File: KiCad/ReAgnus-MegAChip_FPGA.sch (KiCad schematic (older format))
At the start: 3 parts, among them J2 Conn_02x05_Odd_Even, U10 AS4C4M16SA, U7 GW1N-UV9LQ144

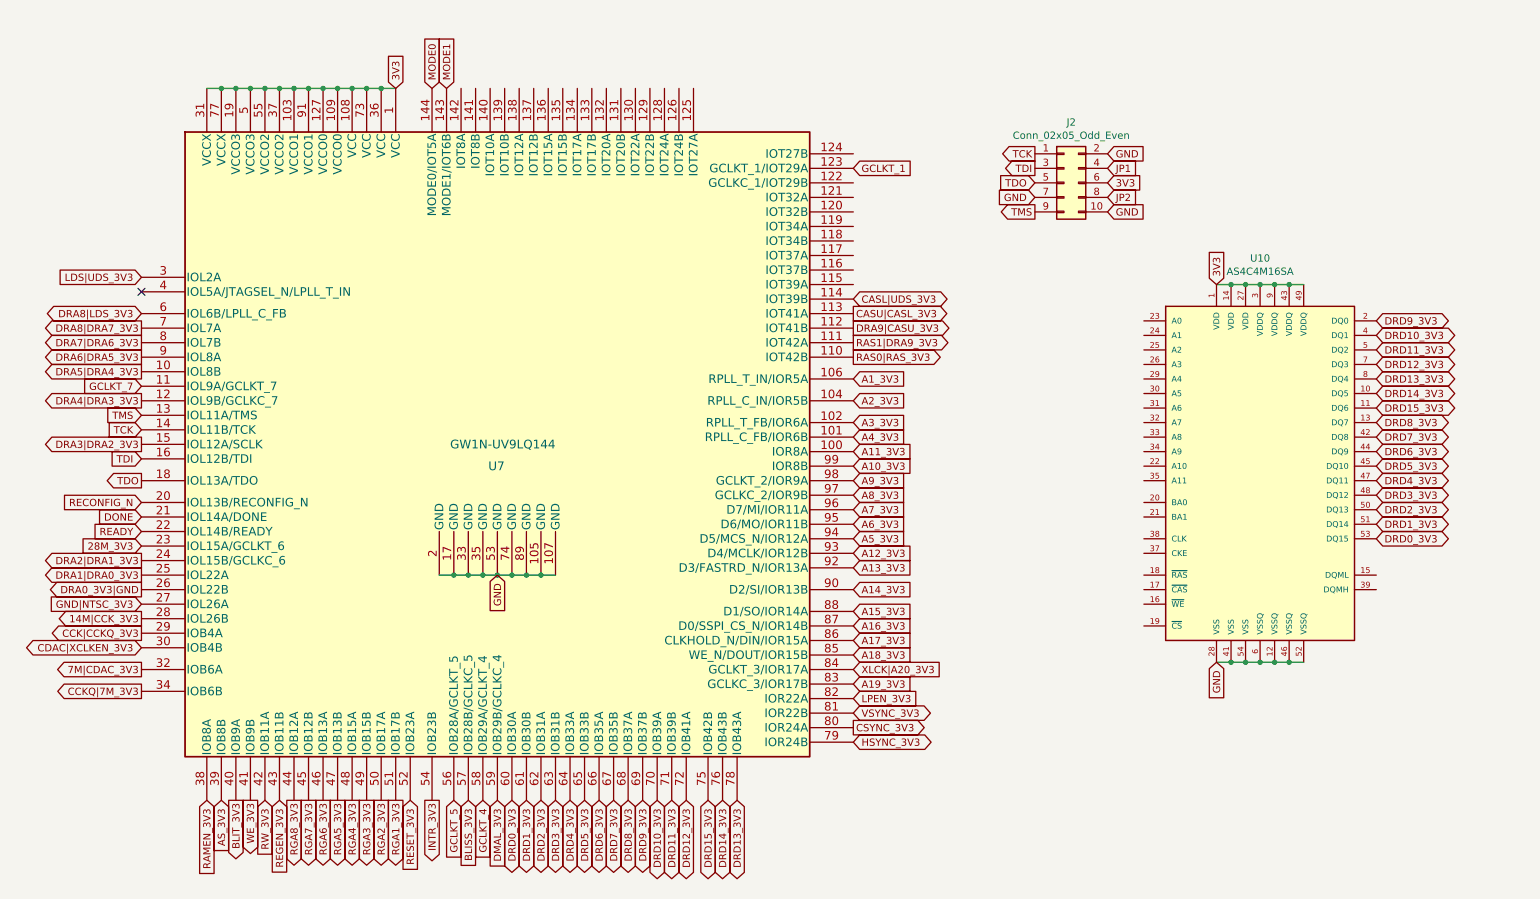
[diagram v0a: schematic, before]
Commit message: more routing and placing components
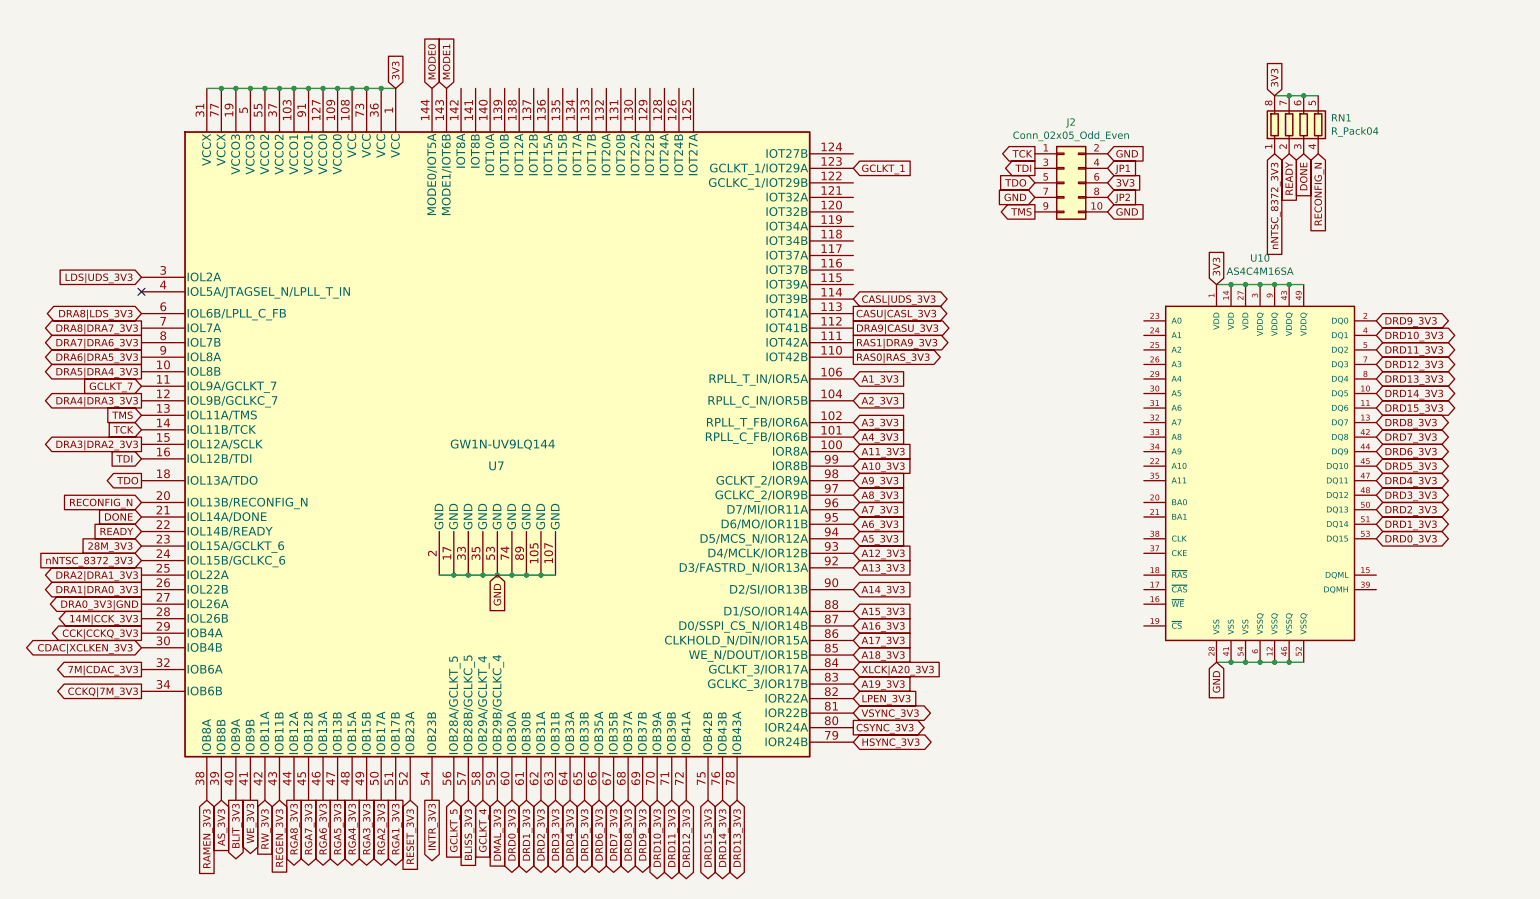
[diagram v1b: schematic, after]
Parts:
- added RN1: R_Pack04, Agnus:RESCAF80P320X160X60-8N, symbol Device:R_Pack04
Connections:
- net GND|NTSC_3V3 is gone; now on net DRA0_3V3|GND: U7.27 (IOL26A)
- net 3V3: now also RN1.5 (R4.2), RN1.6 (R3.2), RN1.7 (R2.2), RN1.8 (R1.2)
- net DONE: now also RN1.3 (R3.1)
- net DRA0_3V3|GND: no longer U7.26 (IOL22B)
- net DRA1|DRA0_3V3: now also U7.26 (IOL22B); no longer U7.25 (IOL22A)
- net DRA2|DRA1_3V3: now also U7.25 (IOL22A); no longer U7.24 (IOL15B/GCLKC_6)
- net READY: now also RN1.2 (R2.1)
- net RECONFIG_N: now also RN1.4 (R4.1)
- new net nNTSC_8372_3V3: RN1.1 (R1.1), U7.24 (IOL15B/GCLKC_6)
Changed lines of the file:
@@
 Text GLabel 5350 5950 3    50   BiDi ~ 0
 DRD15_3V3
-Text GLabel 1450 4600 0    50   Input ~ 0
-GND|NTSC_3V3
 Text GLabel 6350 4950 2    50   Input ~ 0
 A18_3V3
@@
 Text GLabel 1450 3500 0    50   Output ~ 0
 DRA3|DRA2_3V3
-Text GLabel 1450 4300 0    50   Output ~ 0
+Text GLabel 1450 4400 0    50   Output ~ 0
 DRA2|DRA1_3V3
-Text GLabel 1450 4400 0    50   Output ~ 0
+Text GLabel 1450 4500 0    50   Output ~ 0
 DRA1|DRA0_3V3
-Text GLabel 1450 4500 0    50   Output ~ 0
+Text GLabel 1450 4600 0    50   Output ~ 0
 DRA0_3V3|GND
 Text GLabel 2100 5950 3    50   Output ~ 0
@@
 Wire Wire Line
 	9350 5000 9450 5000
+Text GLabel 1450 4300 0    50   Input ~ 0
+nNTSC_8372_3V3
+$Comp
+L Device:R_Pack04 RN1
+U 1 1 6329F720
+P 9450 1300
+F 0 "RN1" H 9638 1346 50  0000 L CNN
+F 1 "R_Pack04" H 9638 1255 50  0000 L CNN
+F 2 "Agnus:RESCAF80P320X160X60-8N" V 9725 1300 50  0001 C CNN
+F 3 "~" H 9450 1300 50  0001 C CNN
+	1    9450 1300
+	1    0    0    -1
+$EndComp
+Text GLabel 9250 1100 1    50   Input ~ 0
+3V3
+Wire Wire Line
+	9250 1100 9350 1100
+Connection ~ 9350 1100
+Wire Wire Line
+	9350 1100 9450 1100
+Connection ~ 9450 1100
+Wire Wire Line
+	9450 1100 9550 1100
+Text GLabel 9550 1500 3    50   Input ~ 0
+RECONFIG_N
+Text GLabel 9450 1500 3    50   Input ~ 0
+DONE
+Text GLabel 9350 1500 3    50   Input ~ 0
+READY
+Text GLabel 9250 1500 3    50   Input ~ 0
+nNTSC_8372_3V3
 $EndSCHEMATC

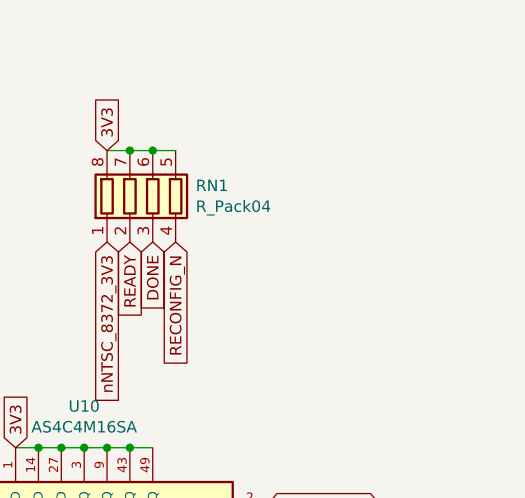
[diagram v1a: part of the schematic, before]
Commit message: more routing and placing components
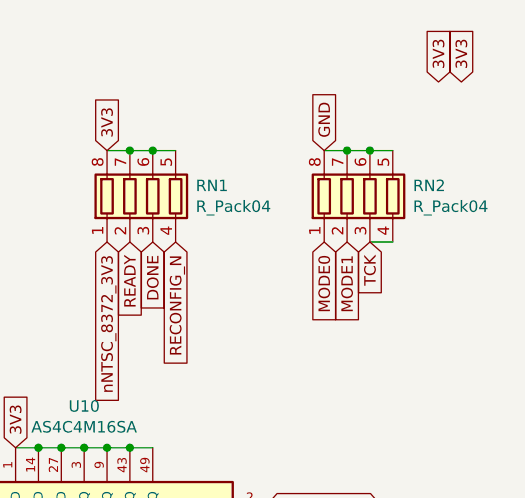
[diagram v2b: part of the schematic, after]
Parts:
- added RN2: R_Pack04, Agnus:RESCAF80P320X160X60-8N, symbol Device:R_Pack04
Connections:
- net GND: now also RN2.5 (R4.2), RN2.6 (R3.2), RN2.7 (R2.2), RN2.8 (R1.2)
- net MODE0: now also RN2.1 (R1.1)
- net MODE1: now also RN2.2 (R2.1)
- net TCK: now also RN2.3 (R3.1), RN2.4 (R4.1)
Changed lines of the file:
@@
 Text GLabel 9250 1500 3    50   Input ~ 0
 nNTSC_8372_3V3
+Text GLabel 10200 1100 1    50   Input ~ 0
+GND
+Text GLabel 10300 1500 3    50   Input ~ 0
+MODE1
+Text GLabel 10200 1500 3    50   Input ~ 0
+MODE0
+Text GLabel 10800 800  1    50   Input ~ 0
+3V3
+$Comp
+L Device:R_Pack04 RN2
+U 1 1 63318369
+P 10400 1300
+F 0 "RN2" H 10588 1346 50  0000 L CNN
+F 1 "R_Pack04" H 10588 1255 50  0000 L CNN
+F 2 "Agnus:RESCAF80P320X160X60-8N" V 10675 1300 50  0001 C CNN
+F 3 "~" H 10400 1300 50  0001 C CNN
+	1    10400 1300
+	1    0    0    -1
+$EndComp
+Text GLabel 10700 800  1    50   Input ~ 0
+3V3
+Wire Wire Line
+	10200 1100 10300 1100
+Connection ~ 10300 1100
+Wire Wire Line
+	10300 1100 10400 1100
+Connection ~ 10400 1100
+Wire Wire Line
+	10400 1100 10500 1100
+Text GLabel 10400 1500 3    50   Input ~ 0
+TCK
+Wire Wire Line
+	10400 1500 10500 1500
 $EndSCHEMATC
